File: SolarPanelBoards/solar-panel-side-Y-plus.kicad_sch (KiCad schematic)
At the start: 56 parts, among them J1 Conn_01x06, U1 OPT3001DNPT

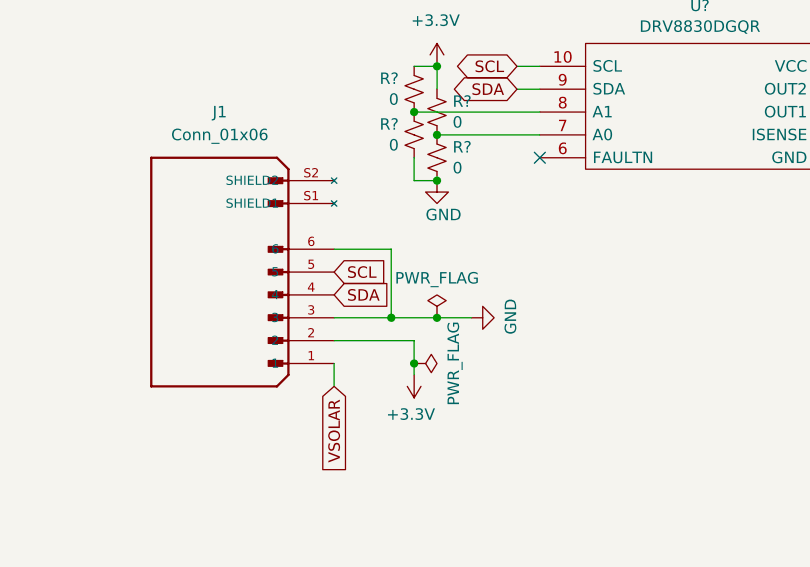
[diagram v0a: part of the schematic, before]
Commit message: updated sch
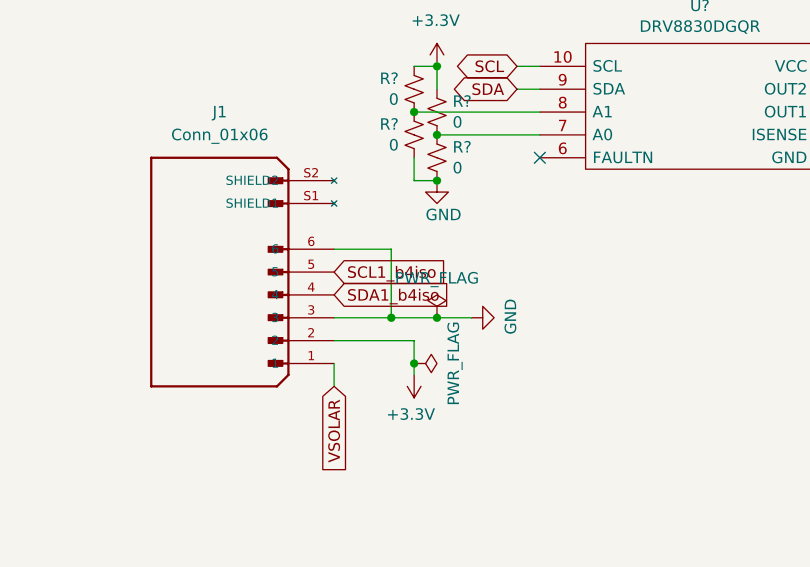
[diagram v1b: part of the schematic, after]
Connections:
- net SCL: no longer J1.5
- net SCL1_b4iso: now also J1.5
- net SDA: no longer J1.4
- net SDA1_b4iso: now also J1.4
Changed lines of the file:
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@@
     )
   )
-  (global_label "SCL" (shape input) (at 167.64 125.73 0) (fields_autoplaced)
+  (global_label "SCL1_b4iso" (shape input) (at 167.64 125.73 0) (fields_autoplaced)
     (effects (font (size 1.27 1.27)) (justify left))
-    (property "Intersheet References" "${INTERSHEET_REFS}" (id 0) (at 0 0 0)
-      (effects (font (size 1.27 1.27)) hide)
+    (property "Intersheet References" "${INTERSHEET_REFS}" (id 0) (at 180.7894 125.6506 0)
+      (effects (font (size 1.27 1.27)) (justify left) hide)
     )
   )
@@
     )
   )
-  (global_label "SDA" (shape input) (at 167.64 128.27 0) (fields_autoplaced)
+  (global_label "SDA1_b4iso" (shape input) (at 167.64 128.27 0) (fields_autoplaced)
     (effects (font (size 1.27 1.27)) (justify left))
-    (property "Intersheet References" "${INTERSHEET_REFS}" (id 0) (at 0 0 0)
-      (effects (font (size 1.27 1.27)) hide)
+    (property "Intersheet References" "${INTERSHEET_REFS}" (id 0) (at 180.8499 128.1906 0)
+      (effects (font (size 1.27 1.27)) (justify left) hide)
     )
   )
